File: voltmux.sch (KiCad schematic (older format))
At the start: 32 parts, among them J5 Conn_02x07_Counter_Clockwise, U10 CD74HC4067SM

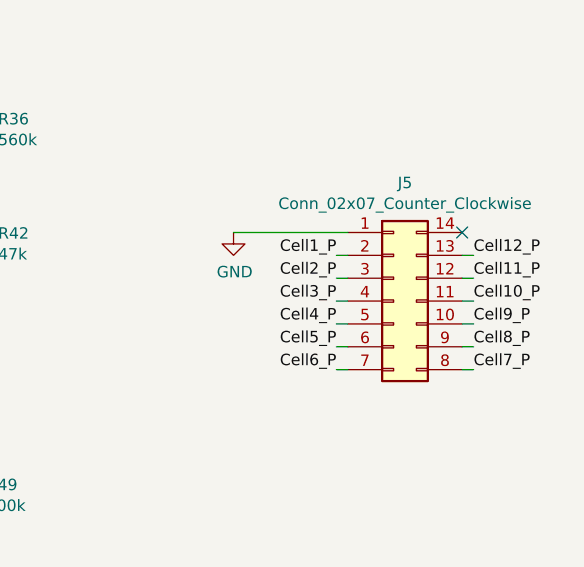
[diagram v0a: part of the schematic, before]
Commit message: routed and filled a bunch of stuff, so much more to do
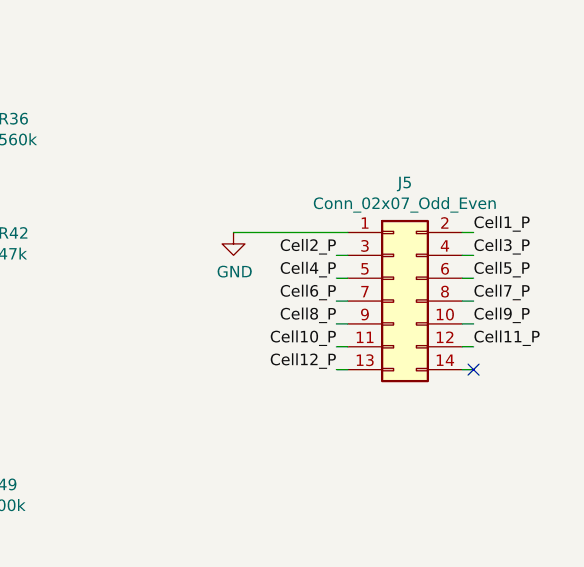
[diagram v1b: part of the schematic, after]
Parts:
- removed J5: Conn_02x07_Counter_Clockwise, uBMS-2:Molex_Milli_Grid_0878325623, symbol Connector_Generic:Conn_02x07_Counter_Clockwise
- added J5: Conn_02x07_Odd_Even, uBMS-2:Molex_Milli_Grid_0878325623_TopBottom, symbol Connector_Generic:Conn_02x07_Odd_Even
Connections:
- net Cell10_P: now also J5.11 (Pin_11)
- net Cell11_P: now also J5.12 (Pin_12)
- net Cell12_P: now also J5.13 (Pin_13)
- net Cell1_P: now also J5.2 (Pin_2)
- net Cell2_P: now also J5.3 (Pin_3)
- net Cell3_P: now also J5.4 (Pin_4)
- net Cell4_P: now also J5.5 (Pin_5)
- net Cell5_P: now also J5.6 (Pin_6)
- net Cell6_P: now also J5.7 (Pin_7)
- net Cell7_P: now also J5.8 (Pin_8)
- net Cell8_P: now also J5.9 (Pin_9)
- net Cell9_P: now also J5.10 (Pin_10)
- net GND: now also J5.1 (Pin_1)
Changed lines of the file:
@@
 	1    0    0    -1
 $EndComp
+Text Label 10450 2100 0    50   ~ 0
+Cell1_P
 Text Label 9850 2200 2    50   ~ 0
-Cell1_P
+Cell2_P
+Text Label 10450 2200 0    50   ~ 0
+Cell3_P
 Text Label 9850 2300 2    50   ~ 0
-Cell2_P
+Cell4_P
+Text Label 10450 2300 0    50   ~ 0
+Cell5_P
 Text Label 9850 2400 2    50   ~ 0
-Cell3_P
+Cell6_P
+Wire Wire Line
+	9400 2100 9900 2100
+Text Label 10450 2400 0    50   ~ 0
+Cell7_P
 Text Label 9850 2500 2    50   ~ 0
-Cell4_P
-Text Label 9850 2600 2    50   ~ 0
-Cell5_P
-Text Label 9850 2700 2    50   ~ 0
-Cell6_P
-$Comp
-L Connector_Generic:Conn_02x07_Counter_Clockwise J5
-U 1 1 5F55EF88
-P 10100 2400
-F 0 "J5" H 10150 2917 50  0000 C CNN
-F 1 "Conn_02x07_Counter_Clockwise" H 10150 2826 50  0000 C CNN
-F 2 "uBMS-2:Molex_Milli_Grid_0878325623" H 10100 2400 50  0001 C CNN
-F 3 "~" H 10100 2400 50  0001 C CNN
-	1    10100 2400
-	1    0    0    -1
-$EndComp
-Wire Wire Line
-	9400 2100 9900 2100
-Text Label 10450 2700 0    50   ~ 0
-Cell7_P
-Text Label 10450 2600 0    50   ~ 0
 Cell8_P
 Text Label 10450 2500 0    50   ~ 0
 Cell9_P
-Text Label 10450 2400 0    50   ~ 0
+Text Label 9850 2600 2    50   ~ 0
 Cell10_P
-Text Label 10450 2300 0    50   ~ 0
+Text Label 10450 2600 0    50   ~ 0
 Cell11_P
-Text Label 10450 2200 0    50   ~ 0
+Text Label 9850 2700 2    50   ~ 0
 Cell12_P
 Wire Wire Line
@@
 Wire Wire Line
 	10450 2200 10400 2200
-NoConn ~ 10400 2100
 Text Label 2900 1650 0    50   ~ 0
 Cell1_P
@@
 Wire Wire Line
 	1800 2950 1850 2950
+$Comp
+L Connector_Generic:Conn_02x07_Odd_Even J5
+U 1 1 5F37E464
+P 10100 2400
+F 0 "J5" H 10150 2917 50  0000 C CNN
+F 1 "Conn_02x07_Odd_Even" H 10150 2826 50  0000 C CNN
+F 2 "uBMS-2:Molex_Milli_Grid_0878325623_TopBottom" H 10100 2400 50  0001 C CNN
+F 3 "~" H 10100 2400 50  0001 C CNN
+	1    10100 2400
+	1    0    0    -1
+$EndComp
+Wire Wire Line
+	10450 2100 10400 2100
+NoConn ~ 10450 2700
 $EndSCHEMATC
